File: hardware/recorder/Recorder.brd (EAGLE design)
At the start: 72.6 x 77.2 mm, 41 parts, among them U1 MCP4822-E/P, U2 LM6132BIN, U3 Value, U4 L7908CV, U5 L7808ABV, U6 ZVN4424A, U7 ZVN4424A, U8 DEV-16771_REDUCED_PINS

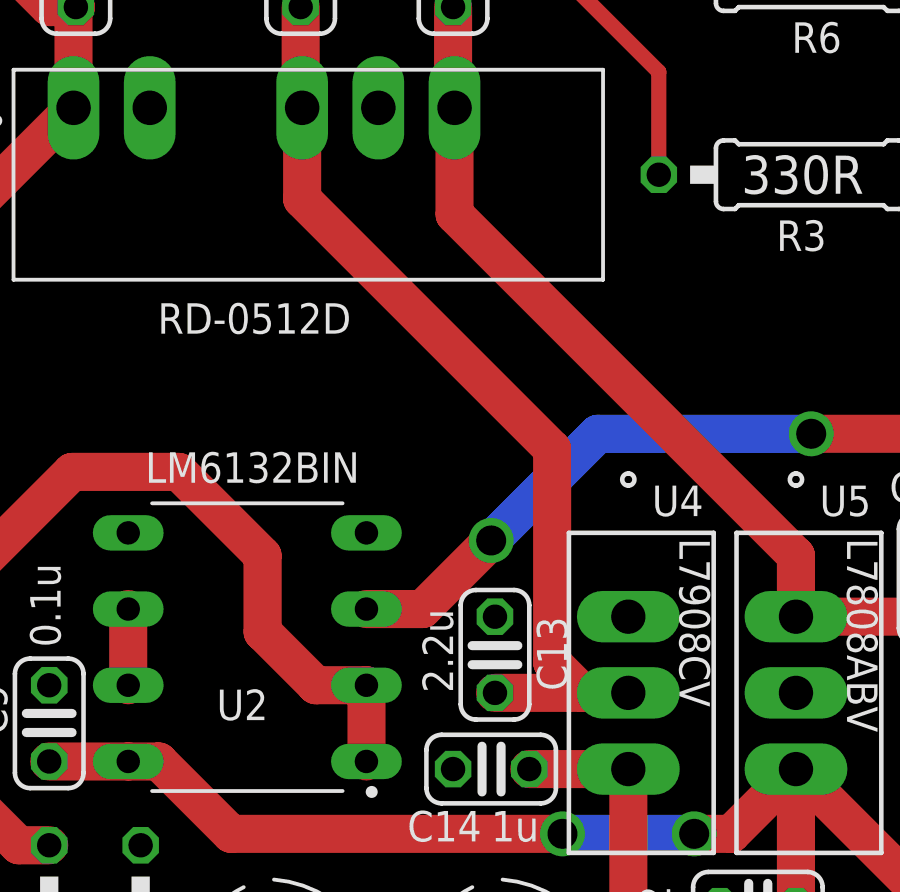
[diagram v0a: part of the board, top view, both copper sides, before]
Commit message: Add minor changes to the hardware
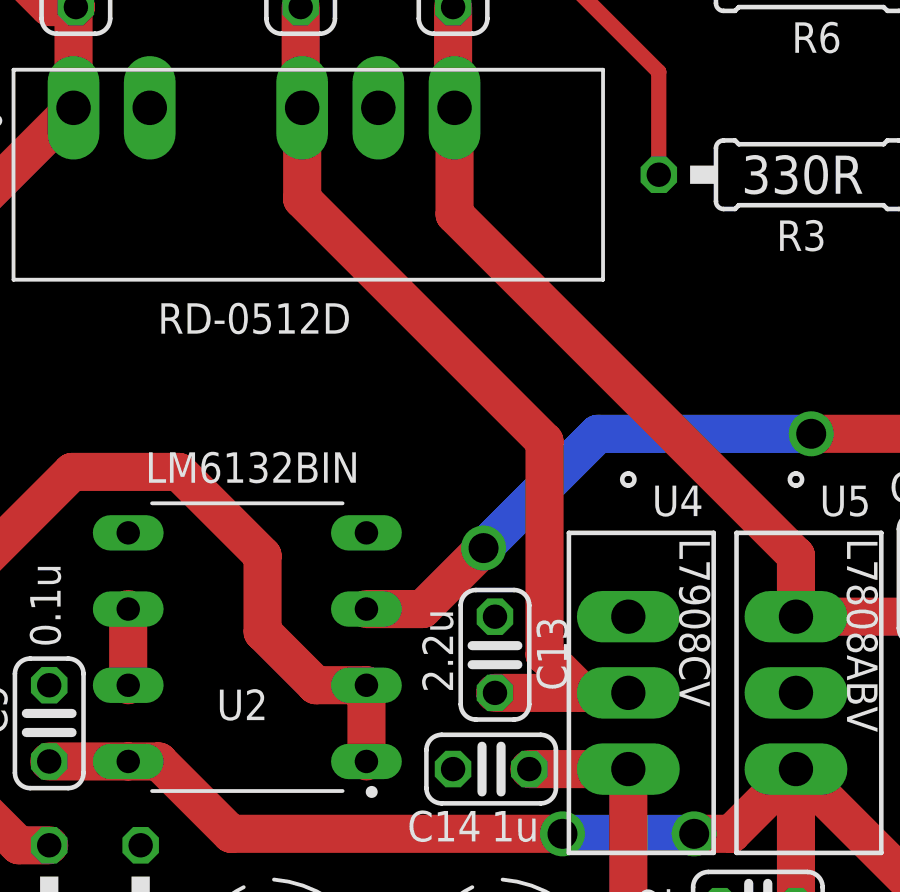
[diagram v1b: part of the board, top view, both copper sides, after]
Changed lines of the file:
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@@
 <via x="51.816" y="50.8" extent="1-16" drill="1"/>
 <wire x1="51.816" y1="50.8" x2="44.704" y2="50.8" width="1.27" layer="16"/>
-<wire x1="44.704" y1="50.8" x2="41.148" y2="47.244" width="1.27" layer="16"/>
-<via x="41.148" y="47.244" extent="1-16" drill="1"/>
-<wire x1="41.148" y1="47.244" x2="38.862" y2="44.958" width="1.27" layer="1"/>
+<wire x1="44.704" y1="50.8" x2="40.894" y2="46.99" width="1.27" layer="16"/>
+<via x="40.894" y="46.99" extent="1-16" drill="1"/>
+<wire x1="40.894" y1="46.99" x2="38.862" y2="44.958" width="1.27" layer="1"/>
 <wire x1="38.862" y1="44.958" x2="36.99" y2="44.958" width="1.27" layer="1"/>
 <wire x1="49.276" y1="27.94" x2="50.8" y2="27.94" width="1.27" layer="1"/>
@@
 <wire x1="34.798" y1="61.715" x2="34.847" y2="61.666" width="1.27" layer="1"/>
 <wire x1="34.847" y1="61.666" x2="34.847" y2="58.625" width="1.27" layer="1"/>
-<wire x1="43.18" y1="43.18" x2="44.196" y2="42.164" width="1.27" layer="1"/>
+<wire x1="42.926" y1="43.434" x2="44.196" y2="42.164" width="1.27" layer="1"/>
 <wire x1="44.196" y1="42.164" x2="45.72" y2="42.164" width="1.27" layer="1"/>
-<wire x1="34.847" y1="58.625" x2="43.18" y2="50.292" width="1.27" layer="1"/>
-<wire x1="43.18" y1="50.292" x2="43.18" y2="43.18" width="1.27" layer="1"/>
+<wire x1="34.847" y1="58.625" x2="42.926" y2="50.546" width="1.27" layer="1"/>
+<wire x1="42.926" y1="50.546" x2="42.926" y2="43.434" width="1.27" layer="1"/>
 <contactref element="C13" pad="2"/>
 <wire x1="41.275" y1="42.164" x2="45.72" y2="42.164" width="1.27" layer="1"/>
